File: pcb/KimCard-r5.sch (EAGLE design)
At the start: 64 parts, among them U1 XMEGA16A4A, U2 MCP2221-I/SL, U4 24AA128SM

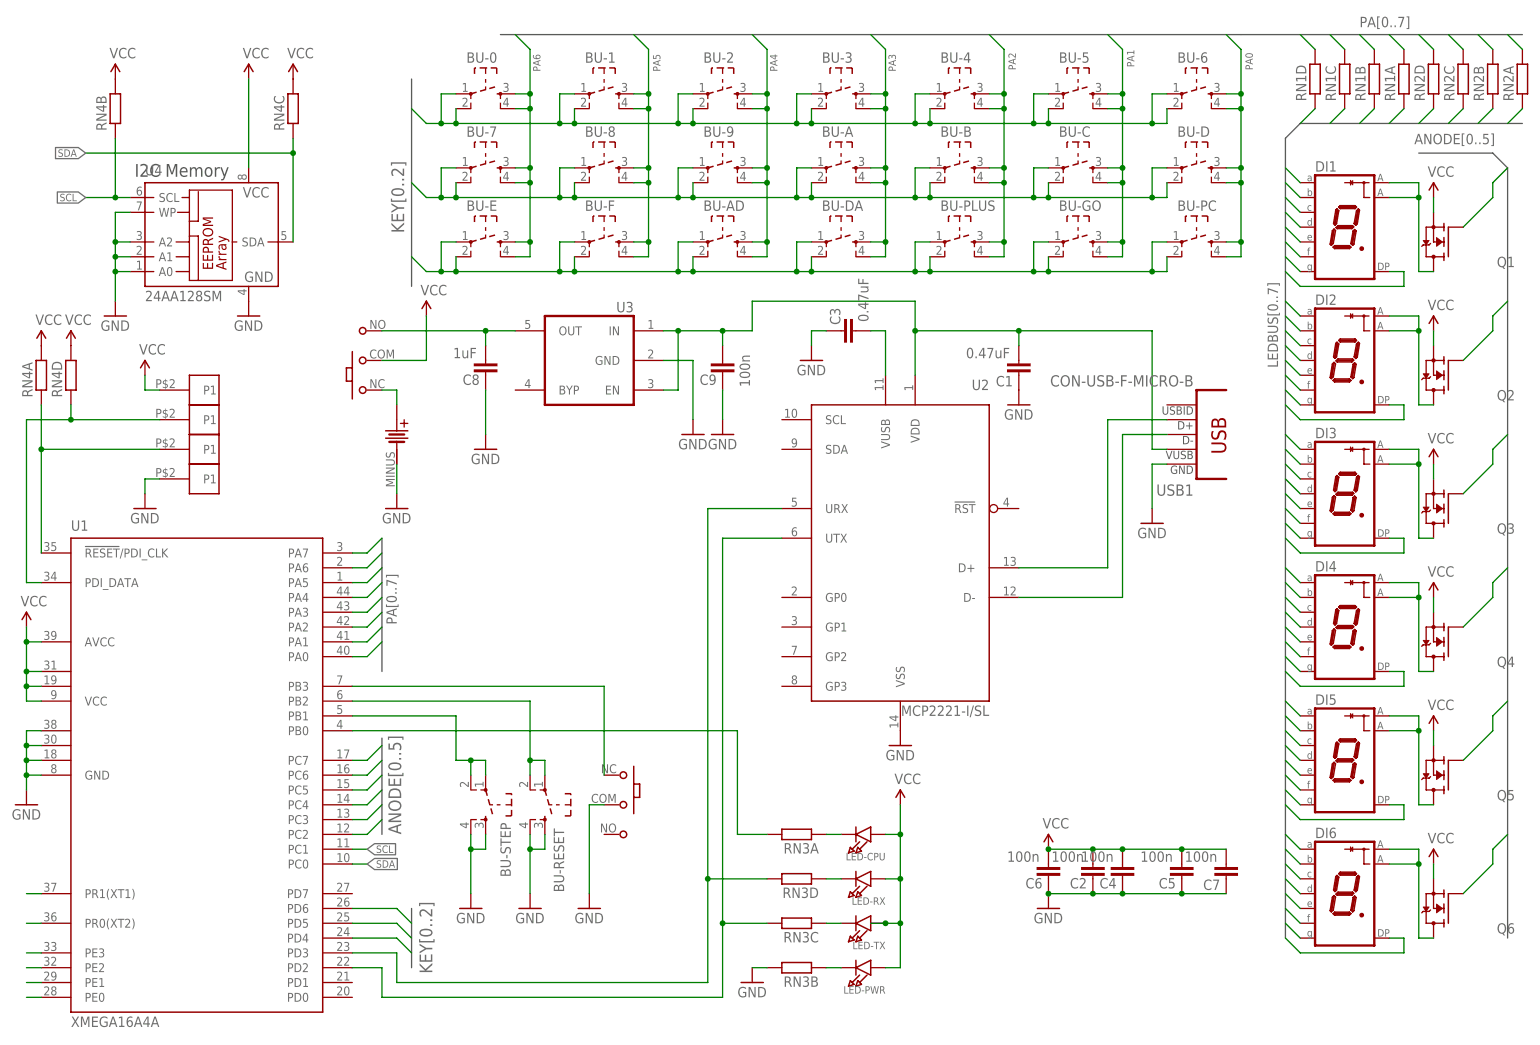
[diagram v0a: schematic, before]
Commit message: Rev 5 almost finalized. Needs silk tuneups
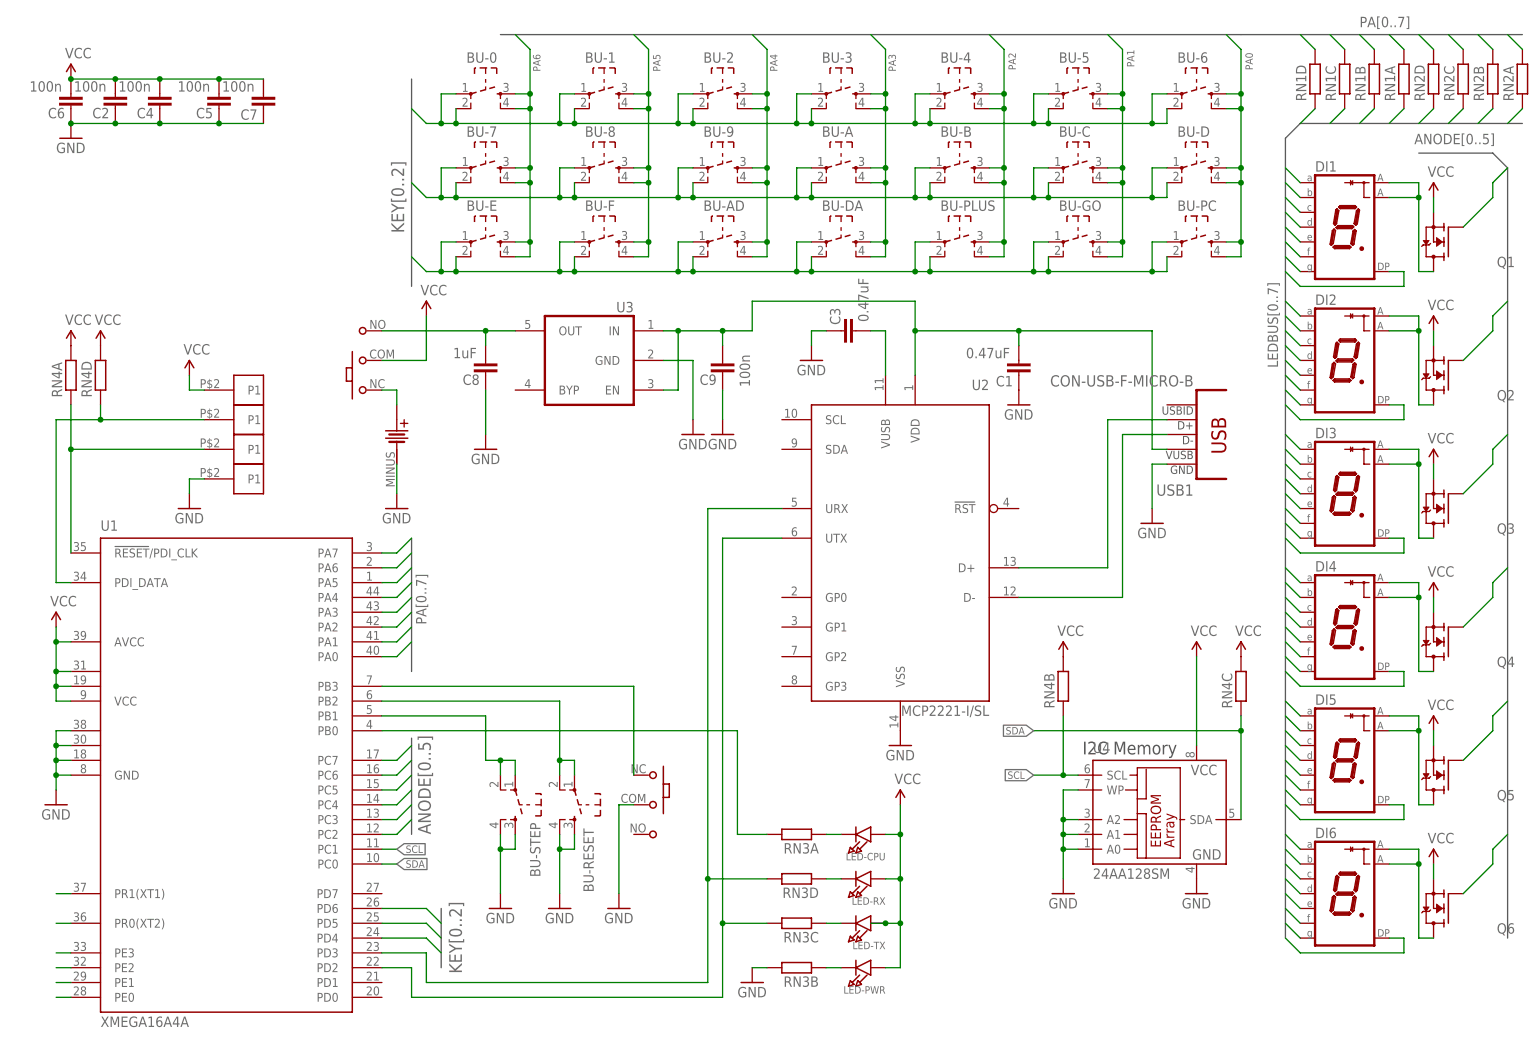
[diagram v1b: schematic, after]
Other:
- moved on the sheet: BU-RESET, BU-STEP, C2, C4, C5, C6, C7, RN4A, RN4B, RN4C, RN4D, U1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
